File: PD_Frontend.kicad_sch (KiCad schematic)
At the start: 17 parts, among them U2 TPS2372

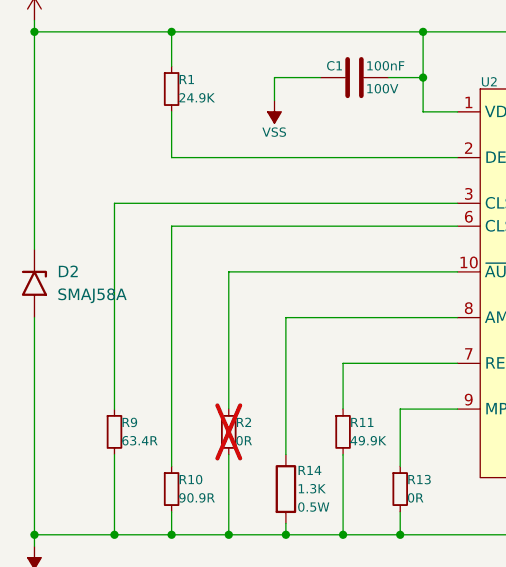
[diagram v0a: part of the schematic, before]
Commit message: add ci
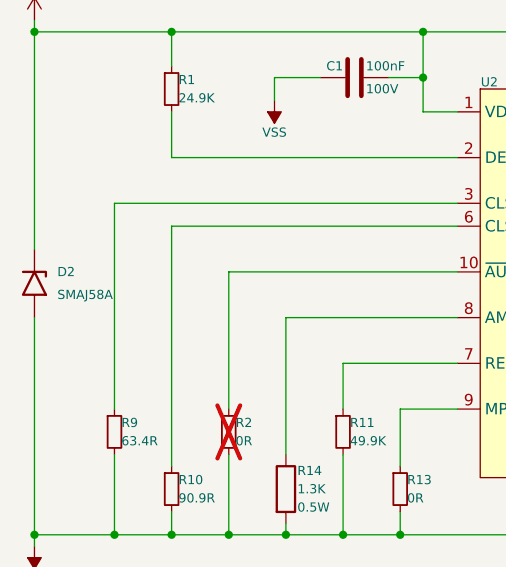
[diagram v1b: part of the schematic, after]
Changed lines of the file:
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@@
 			(effects
 				(font
-					(size 1.27 1.27)
+					(size 1.016 1.016)
 				)
 				(justify left)
@@
 			(effects
 				(font
-					(size 1.27 1.27)
+					(size 1.016 1.016)
 				)
 				(justify left)
